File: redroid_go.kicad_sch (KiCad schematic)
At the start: 100 parts, among them J1 USB4105-GF-A, J2 5051101892, J3 Conn_01x02_Pin, J4 Conn_01x10_Pin, Q1 UMH3N, Q2 PMOS, Q3 UMH3N, SW1 UP, SW10 A, SW11 SW_SPDT, SW2 DOWN, SW3 LEFT, SW4 RIGHT, SW5 MENU, SW6 VOLUME, SW7 SELECT, SW8 START, SW9 B, U1 ESP32-WROVER-E-N16R8, U2 CH340C, U3 MP2161GJ-Z, U4 XC6802A42XMR-G, U5 AMS1117-3.3, U7 NC7SZ125M5X, U8 NC7SZ125M5X, U9 NC7SZ125M5X

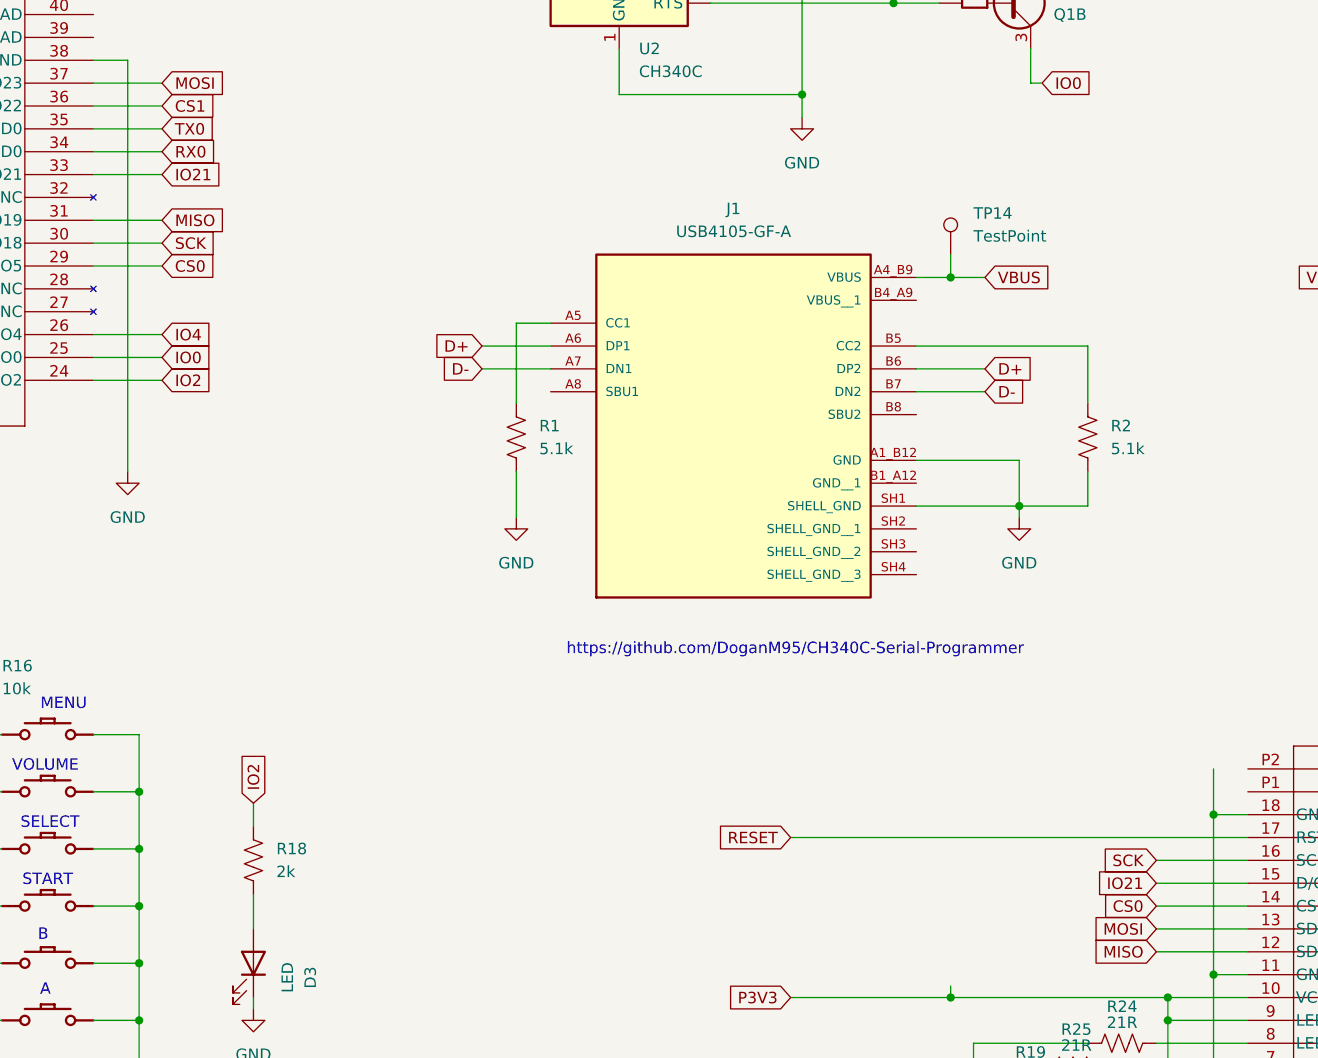
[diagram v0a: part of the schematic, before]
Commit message: Rename label
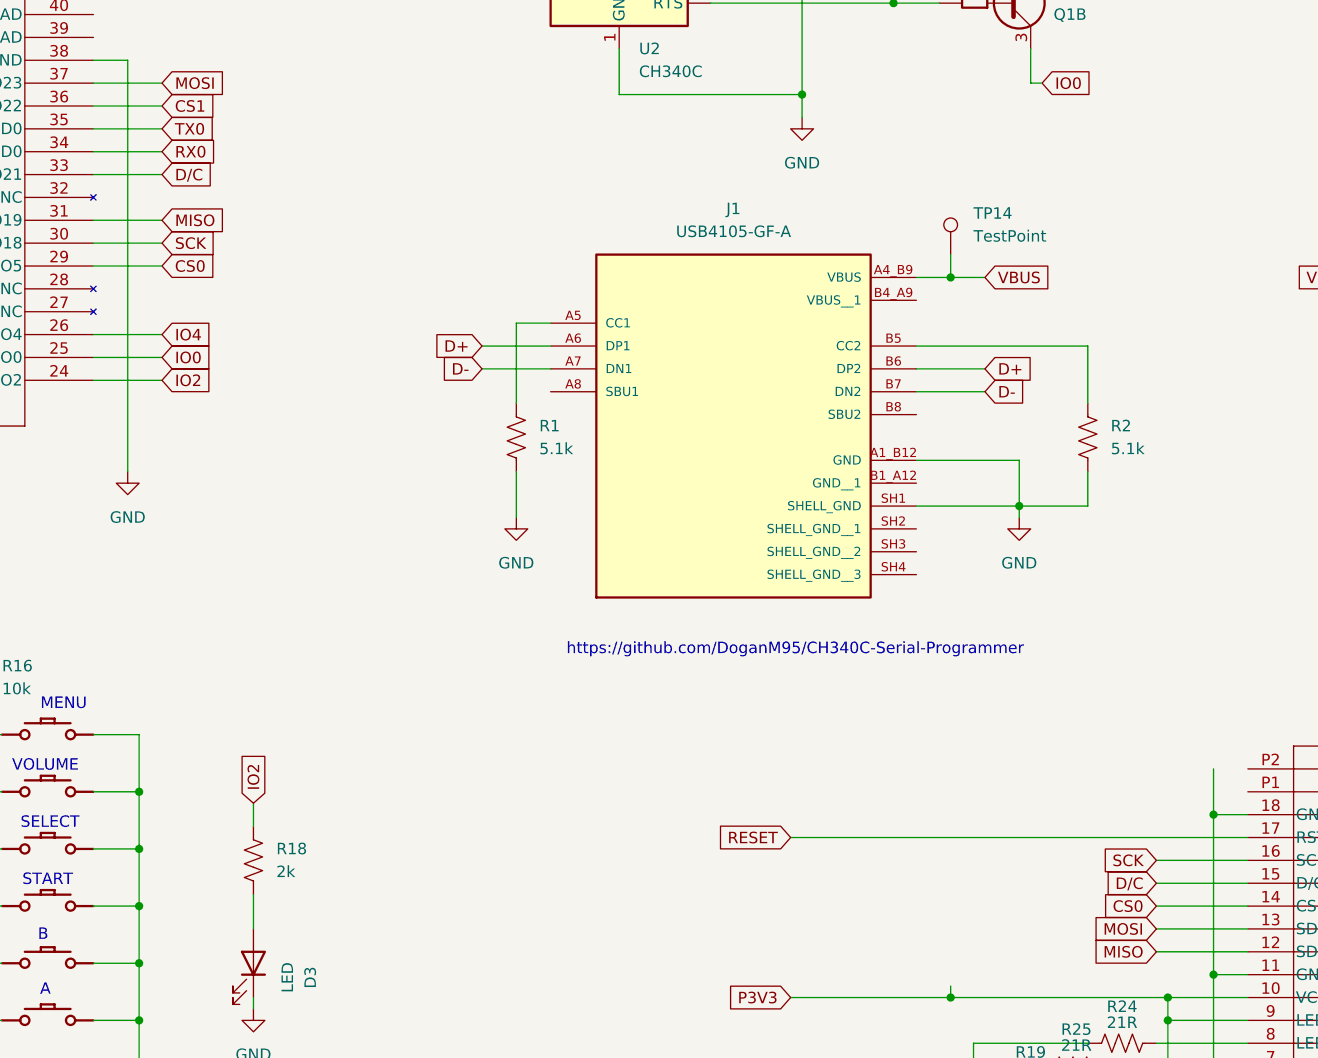
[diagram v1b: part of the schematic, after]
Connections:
- net IO21 renamed D/C
- net D/C: no longer U1.33 (IO21)
- new net D/C: U1.33 (IO21)
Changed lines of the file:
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@@
 		)
 	)
-	(global_label "IO21"
+	(global_label "D/C"
 		(shape input)
 		(at 240.03 154.94 180)
@@
 		)
 	)
-	(global_label "IO21"
+	(global_label "D{slash}C"
 		(shape input)
 		(at 129.54 76.2 0)
@@
 		)
 		(property "Intersheetrefs" "${INTERSHEET_REFS}"
-			(at 136.8795 76.2 0)
-			(effects
-				(font
+			(at 136.3957 76.2 0)
+			(effects
+				(font
